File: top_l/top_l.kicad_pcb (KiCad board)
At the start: 2 copper layers, 128.4 x 119.3 mm, 31 parts, among them SW29 SW_Push, SW30 SW_Push, SW31 SW_Push, SW32 SW_Push, SW33 SW_Push, SW34 SW_Push, SW35 SW_Push, SW36 SW_Push, SW37 SW_Push, SW38 SW_Push, SW39 SW_Push, SW40 SW_Push, SW41 SW_Push, SW42 SW_Push, SW43 SW_Push, SW44 SW_Push, SW45 SW_Push, SW46 SW_Push, SW47 SW_Push, SW48 SW_Push, SW49 SW_Push, SW50 SW_Push, SW51 SW_Push, SW52 SW_Push, SW53 SW_Push, SW54 SW_Push, SW55 SW_Push

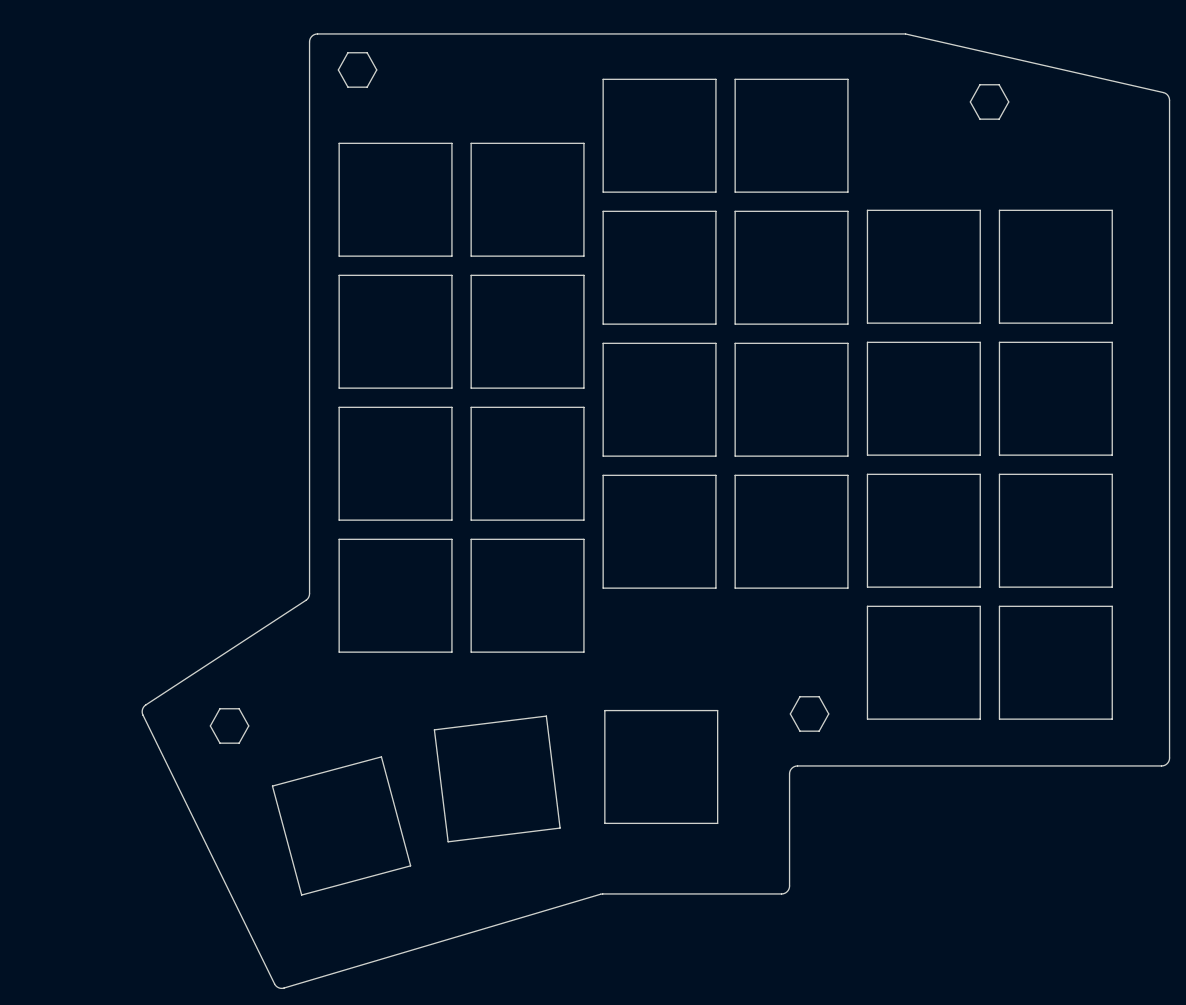
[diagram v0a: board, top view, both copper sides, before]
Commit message: feat: add switch plate
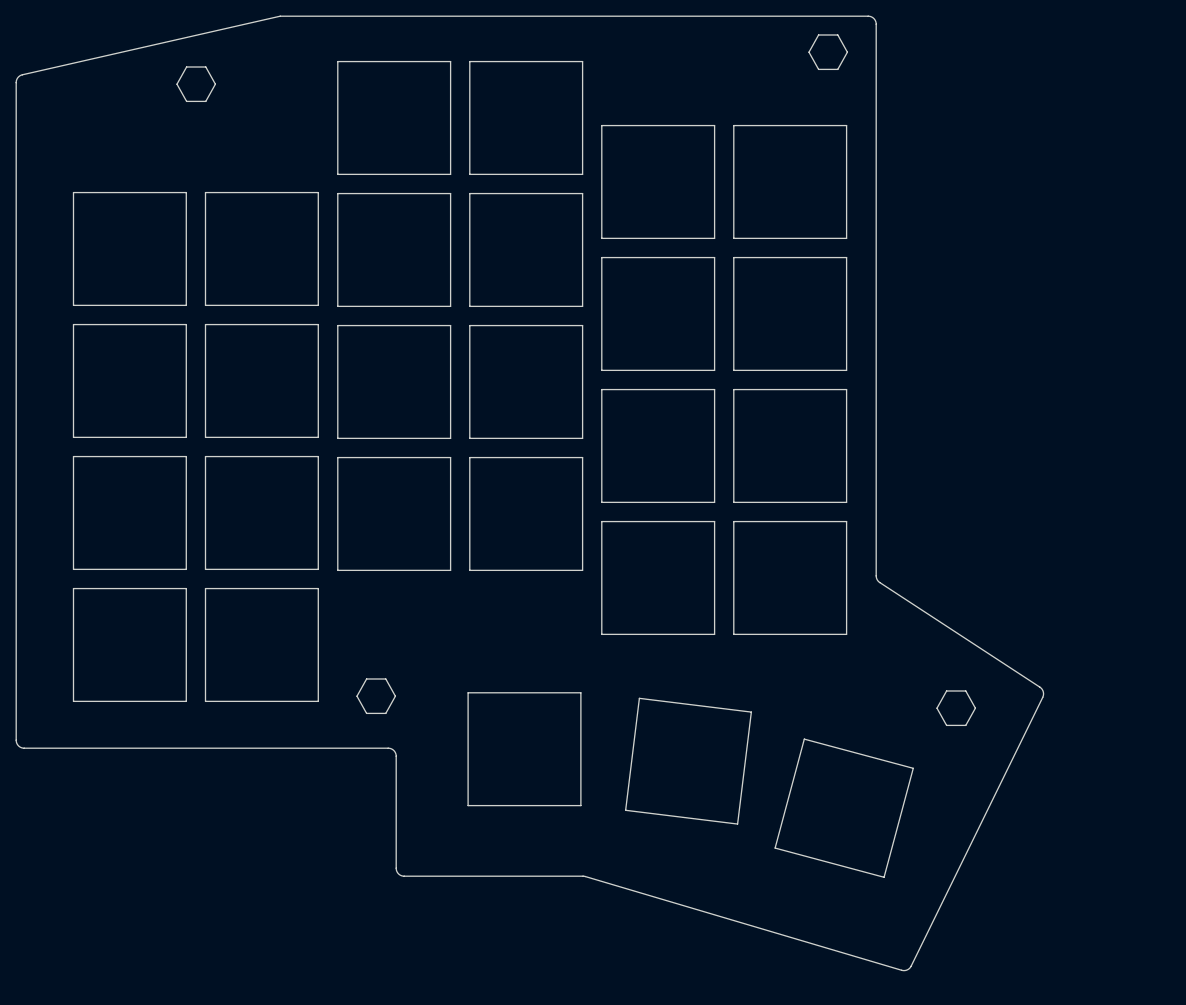
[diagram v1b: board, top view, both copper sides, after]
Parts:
- moved SW52 115.8 mm to (86.0, 66.9)
- moved SW53 115.8 mm to (86.0, 83.4)
- moved SW54 115.8 mm to (86.0, 99.9)
- moved SW55 115.8 mm to (86.0, 116.4)
- moved Ref** 99.2 mm to (94.3, 46.3)
- moved Ref** 90.9 mm to (189.3, 124.3)
- moved SW48 82.8 mm to (102.5, 66.9)
- moved SW49 82.8 mm to (102.5, 83.4)
- moved SW50 82.8 mm to (102.5, 99.9)
- moved SW51 82.8 mm to (102.5, 116.4)
- moved SW33 62.9 mm to (175.3, 136.8), turned to -15 degrees
- moved Ref** 58.9 mm to (173.3, 42.3)
- moved Ref** 54.2 mm to (116.8, 122.8)
- moved SW44 49.7 mm to (119.1, 50.5)
- moved SW45 49.7 mm to (119.1, 67.0)
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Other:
- outline, holes or cut-outs redrawn
